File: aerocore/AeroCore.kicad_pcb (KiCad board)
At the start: 2 copper layers, 75 x 68 mm, 6 parts

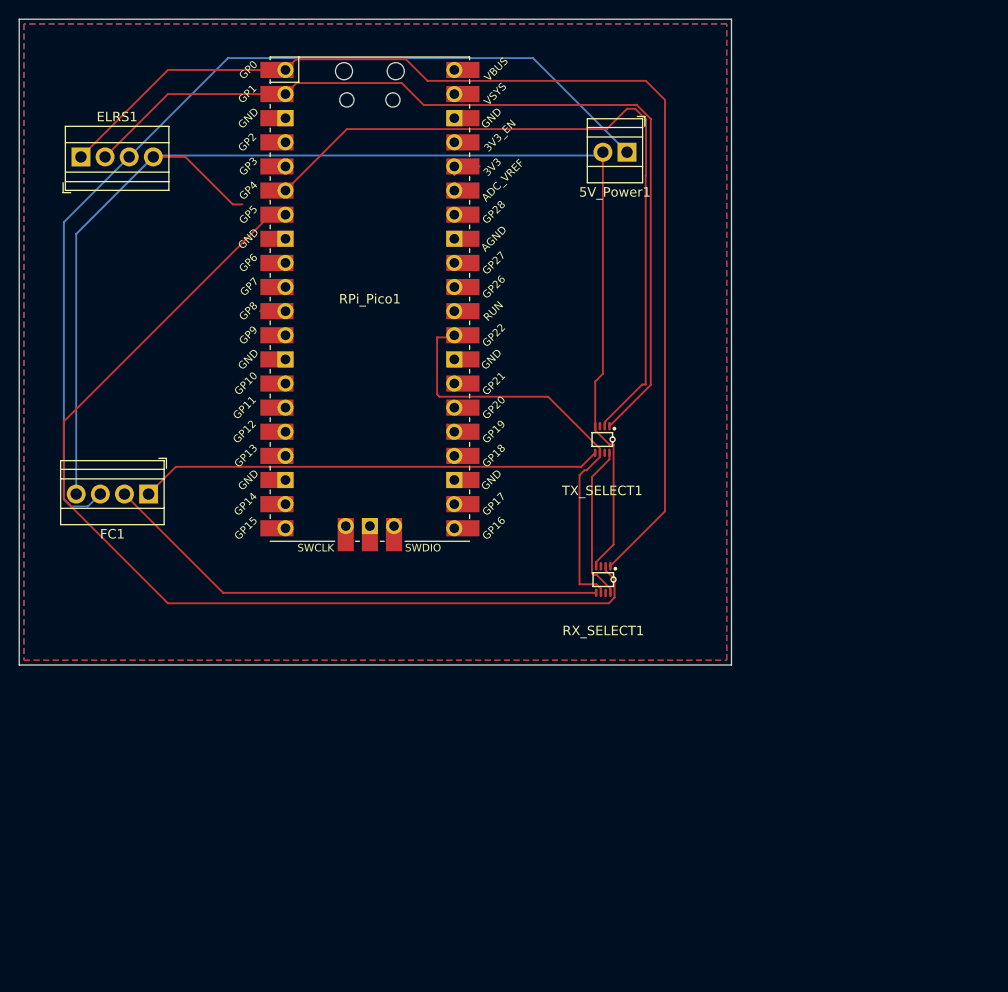
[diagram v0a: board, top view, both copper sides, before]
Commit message: add firmware and pcb
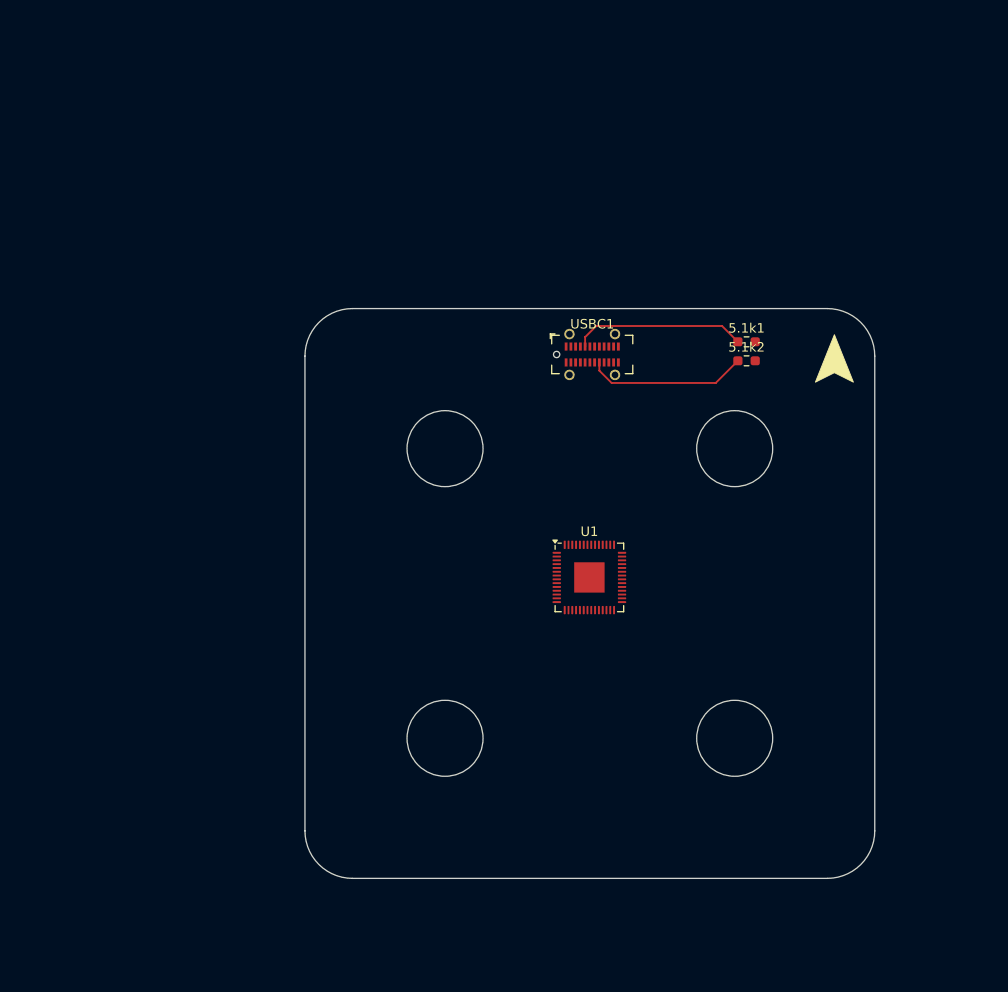
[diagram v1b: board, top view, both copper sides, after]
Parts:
- removed 5V_Power1: Conn_01x02, TerminalBlock:TerminalBlock_Xinya_XY308-2.54-2P_1x02_P2.54mm_Horizontal
- removed ELRS1, FC1: Conn_01x04, TerminalBlock:TerminalBlock_Xinya_XY308-2.54-4P_1x04_P2.54mm_Horizontal
- removed RPi_Pico1: Pico, RPi_Pico:RPi_Pico_SMD_TH
- removed RX_SELECT1, TX_SELECT1: SN74LVC2G157DCUR, easyeda2kicad:VSSOP-8_L2.3-W2.0-P0.50-LS3.1-BL
- added 5.1k1: 5.1k, Resistor_SMD:R_0603_1608Metric_Pad0.98x0.95mm_HandSolder, F.Cu at (91.5, 48.5)
- added 5.1k2: 5.1k, Resistor_SMD:R_0603_1608Metric_Pad0.98x0.95mm_HandSolder, F.Cu at (91.5, 50.5)
- added U1: RP2040, Package_DFN_QFN:QFN-56-1EP_7x7mm_P0.4mm_EP3.2x3.2mm, F.Cu at (75.0, 73.3)
- added USBC1: USB_C_Receptacle_USB2.0_16P, Connector_USB:USB_C_Receptacle_GCT_USB4115-03-C, F.Cu at (75.2, 49.8)
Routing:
- net /POWER.GND: track 143.6 -> 0.00 mm
- net /UART0.TX: track 119.0 -> 0.00 mm
- net /UART1.RX: track 107.0 -> 0.00 mm
- net /POWER.5V: track 104.4 -> 0.00 mm
- net /UART0.RX: track 96.4 -> 0.00 mm
- net /UART1.TX: track 76.3 -> 0.00 mm
- net /UART_FC.TX: track 54.0 -> 0.00 mm
- net /UART_FC.RX: track 48.8 -> 0.00 mm
- net /SEL: track 45.6 -> 0.00 mm
- net Net-(USBC1-CC1): track 0.00 -> 18.3 mm
- net Net-(USBC1-CC2): track 0.00 -> 17.0 mm
- net /POWER.3V3: track 16.5 -> 0.00 mm
- net unconnected-(RPi_Pico1-3V3-Pad36): track 3.60 -> 0.00 mm
- net unconnected-(RPi_Pico1-GPIO8-Pad11): track 2.67 -> 0.00 mm
- net unconnected-(RPi_Pico1-GND-Pad8): track 2.25 -> 0.00 mm
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- removed copper zone on B.Cu, net /POWER.GND
- removed copper zone on F.Cu, net /POWER.GND
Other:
- board size 75 x 68 mm -> 60 x 60 mm
- board text added: "AeroNode"

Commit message: make custom rp2040 based design
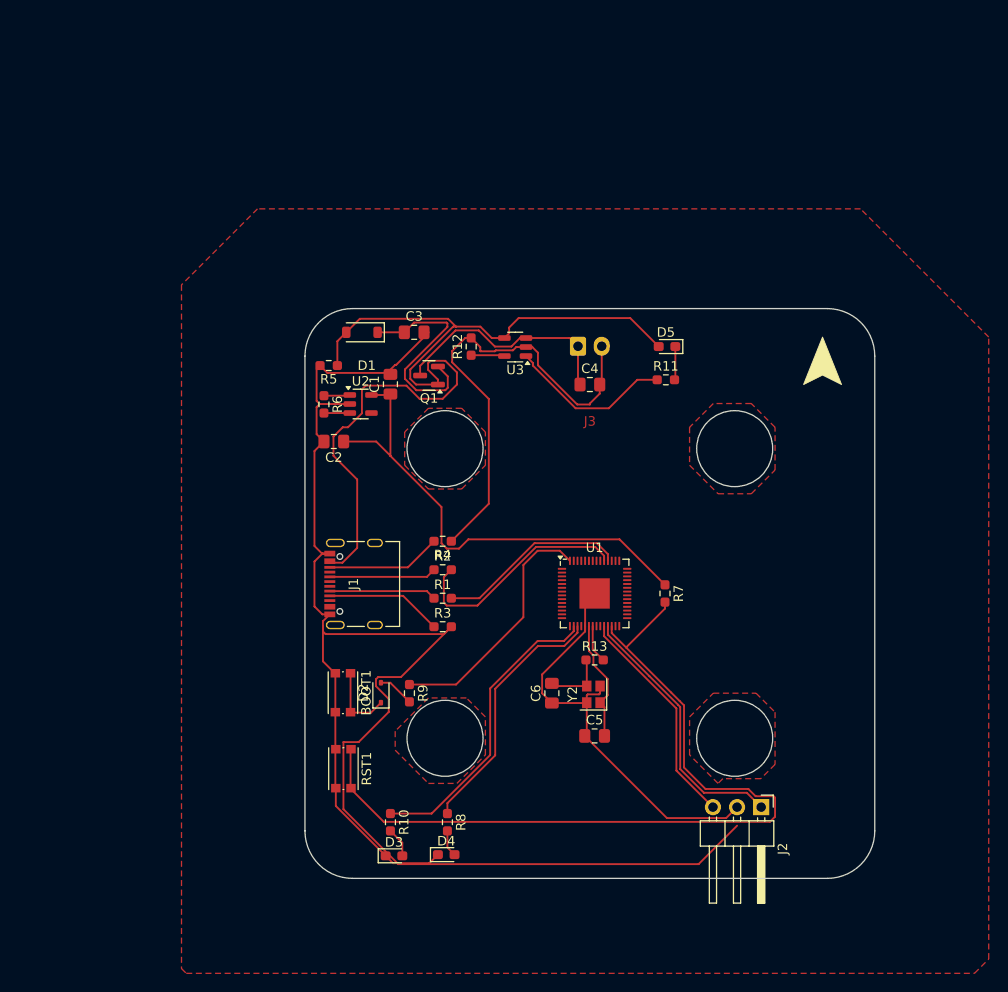
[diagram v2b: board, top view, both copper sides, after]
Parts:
- removed 5.1k1, 5.1k2: 5.1k, Resistor_SMD:R_0603_1608Metric_Pad0.98x0.95mm_HandSolder
- removed USBC1: USB_C_Receptacle_USB2.0_16P, Connector_USB:USB_C_Receptacle_GCT_USB4115-03-C
- added BOOT1: SW_SPST, Button_Switch_SMD:SW_Push_1P1T_NO_CK_KMR2, F.Cu at (49.0, 85.5)
- added C1: 10uF, Capacitor_SMD:C_0805_2012Metric_Pad1.18x1.45mm_HandSolder, F.Cu at (54.0, 53.0)
- added C2: 10uF, Capacitor_SMD:C_0805_2012Metric_Pad1.18x1.45mm_HandSolder, F.Cu at (48.0, 59.0)
- added C3: 10uF, Capacitor_SMD:C_0805_2012Metric_Pad1.18x1.45mm_HandSolder, F.Cu at (56.5, 47.5)
- added C4: 10uF, Capacitor_SMD:C_0805_2012Metric_Pad1.18x1.45mm_HandSolder, F.Cu at (75.0, 53.0)
- added C5: 22pF, Capacitor_SMD:C_0805_2012Metric_Pad1.18x1.45mm_HandSolder, F.Cu at (75.5, 90.0)
- added C6: 22pF, Capacitor_SMD:C_0805_2012Metric_Pad1.18x1.45mm_HandSolder, F.Cu at (71.0, 85.5)
- added D1: MBR0540, Diode_SMD:D_SOD-123, F.Cu at (51.0, 47.5)
- added D2: NSR0340HT1G, Diode_SMD:D_SOD-323, F.Cu at (53.0, 85.5)
- added D3: RED, LED_SMD:LED_0603_1608Metric_Pad1.05x0.95mm_HandSolder, F.Cu at (54.4, 102.6)
- added D4: RED, LED_SMD:LED_0603_1608Metric_Pad1.05x0.95mm_HandSolder, F.Cu at (59.9, 102.5)
- added D5: ORANGE, LED_SMD:LED_0603_1608Metric_Pad1.05x0.95mm_HandSolder, F.Cu at (83.1, 49.0)
- added J1: USB_C_Receptacle_USB2.0_16P, Connector_USB:USB_C_Receptacle_Palconn_UTC16-G, F.Cu at (50.1, 74.0)
- added J2: Conn_01x03_Pin, Connector_PinHeader_2.54mm:PinHeader_1x03_P2.54mm_Horizontal, F.Cu at (93.0, 97.5)
- added J3: Conn_01x02_Pin, Connector_JST:JST_EH_S2B-EH_1x02_P2.50mm_Horizontal, B.Cu at (73.8, 49.0)
- added Q1: DMG3418L, Package_TO_SOT_SMD:SOT-23, F.Cu at (58.1, 52.0)
- added R1: 27, Resistor_SMD:R_0603_1608Metric_Pad0.98x0.95mm_HandSolder, F.Cu at (59.5, 75.5)
- added R10: 10k, Resistor_SMD:R_0603_1608Metric_Pad0.98x0.95mm_HandSolder, F.Cu at (54.0, 99.1)
- added R11: 10k, Resistor_SMD:R_0603_1608Metric_Pad0.98x0.95mm_HandSolder, F.Cu at (83.0, 52.5)
- added R12: 5.1k, Resistor_SMD:R_0603_1608Metric_Pad0.98x0.95mm_HandSolder, F.Cu at (62.5, 49.0)
- added R13: 1k, Resistor_SMD:R_0603_1608Metric_Pad0.98x0.95mm_HandSolder, F.Cu at (75.5, 82.0)
- added R2: 27, Resistor_SMD:R_0603_1608Metric_Pad0.98x0.95mm_HandSolder, F.Cu at (59.5, 72.5)
- added R3: 5.1k, Resistor_SMD:R_0603_1608Metric_Pad0.98x0.95mm_HandSolder, F.Cu at (59.5, 78.5)
- added R4: 5.1k, Resistor_SMD:R_0603_1608Metric_Pad0.98x0.95mm_HandSolder, F.Cu at (59.5, 69.5)
- added R5: 10k, Resistor_SMD:R_0603_1608Metric_Pad0.98x0.95mm_HandSolder, F.Cu at (47.5, 51.0)
- added R6: 10k, Resistor_SMD:R_0603_1608Metric_Pad0.98x0.95mm_HandSolder, F.Cu at (47.0, 55.1)
- added R7: 10k, Resistor_SMD:R_0603_1608Metric_Pad0.98x0.95mm_HandSolder, F.Cu at (82.9, 75.0)
- added R8: 10k, Resistor_SMD:R_0603_1608Metric_Pad0.98x0.95mm_HandSolder, F.Cu at (60.0, 99.1)
- added R9: 1k, Resistor_SMD:R_0603_1608Metric_Pad0.98x0.95mm_HandSolder, F.Cu at (56.0, 85.5)
- added RST1: SW_SPST, Button_Switch_SMD:SW_Push_1P1T_NO_CK_KMR2, F.Cu at (49.0, 93.5)
- added U2: AP2112K-3.3, Package_TO_SOT_SMD:SOT-23-5, F.Cu at (50.9, 55.0)
- added U3: MCP73831-2-OT, Package_TO_SOT_SMD:SOT-23-5, F.Cu at (67.1, 49.0)
- added Y2: 12MHz, Crystal:Crystal_SMD_2520-4Pin_2.5x2.0mm, F.Cu at (75.4, 85.6)
- moved U1 1.77 mm to (75.5, 75.0)
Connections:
- U1 pad 16: unconnected-(U1-GPIO13-Pad16) -> /D13
- U1 pad 17: unconnected-(U1-GPIO14-Pad17) -> /D14
- U1 pad 19: unconnected-(U1-TESTEN-Pad19) -> GND
- U1 pad 20: unconnected-(U1-XIN-Pad20) -> /XIN
- U1 pad 21: unconnected-(U1-XOUT-Pad21) -> /XOUT
- U1 pad 24: unconnected-(U1-SWCLK-Pad24) -> /SWCLK
- U1 pad 25: unconnected-(U1-SWD-Pad25) -> /SWDIO
- U1 pad 26: unconnected-(U1-RUN-Pad26) -> /~{RESET}
- U1 pad 46: unconnected-(U1-USB_DM-Pad46) -> /D-
- U1 pad 47: unconnected-(U1-USB_DP-Pad47) -> /D+
- U1 pad 56: unconnected-(U1-QSPI_SS-Pad56) -> /QSPI_CS
- U1 pad 57: unconnected-(U1-GND-Pad57) -> GND
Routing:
- net GND: track 0.00 -> 263.4 mm
- net /VBUS: track 0.00 -> 93.4 mm
- net /~{RESET}: track 0.00 -> 87.9 mm
- net /+3v3: track 0.00 -> 51.0 mm
- net /D13: track 0.00 -> 31.9 mm
- net /SWDIO: track 0.00 -> 28.4 mm
- net /D14: track 0.00 -> 27.0 mm
- net /QSPI_CS: track 0.00 -> 26.4 mm
- net Net-(D1-K): track 0.00 -> 26.0 mm
- net /VBAT: track 0.00 -> 24.7 mm
- net /D+: track 0.00 -> 24.3 mm
- net /SWCLK: track 0.00 -> 23.8 mm
- net /D-: track 0.00 -> 20.1 mm
- net Net-(USBC1-CC1): track 18.3 -> 0.00 mm
- net Net-(U3-STAT): track 0.00 -> 17.5 mm
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- added copper zone on F.Cu, net GND
